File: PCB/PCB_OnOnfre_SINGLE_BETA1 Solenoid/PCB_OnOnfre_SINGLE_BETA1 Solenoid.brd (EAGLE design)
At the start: 44.1 x 43.8 mm, 32 parts, among them J1 9PIN 2.54MM, J3Y S8050, J7 8p, K1 G5Q-1-DC12, K2 G5Q-1-DC12, U2 esp12

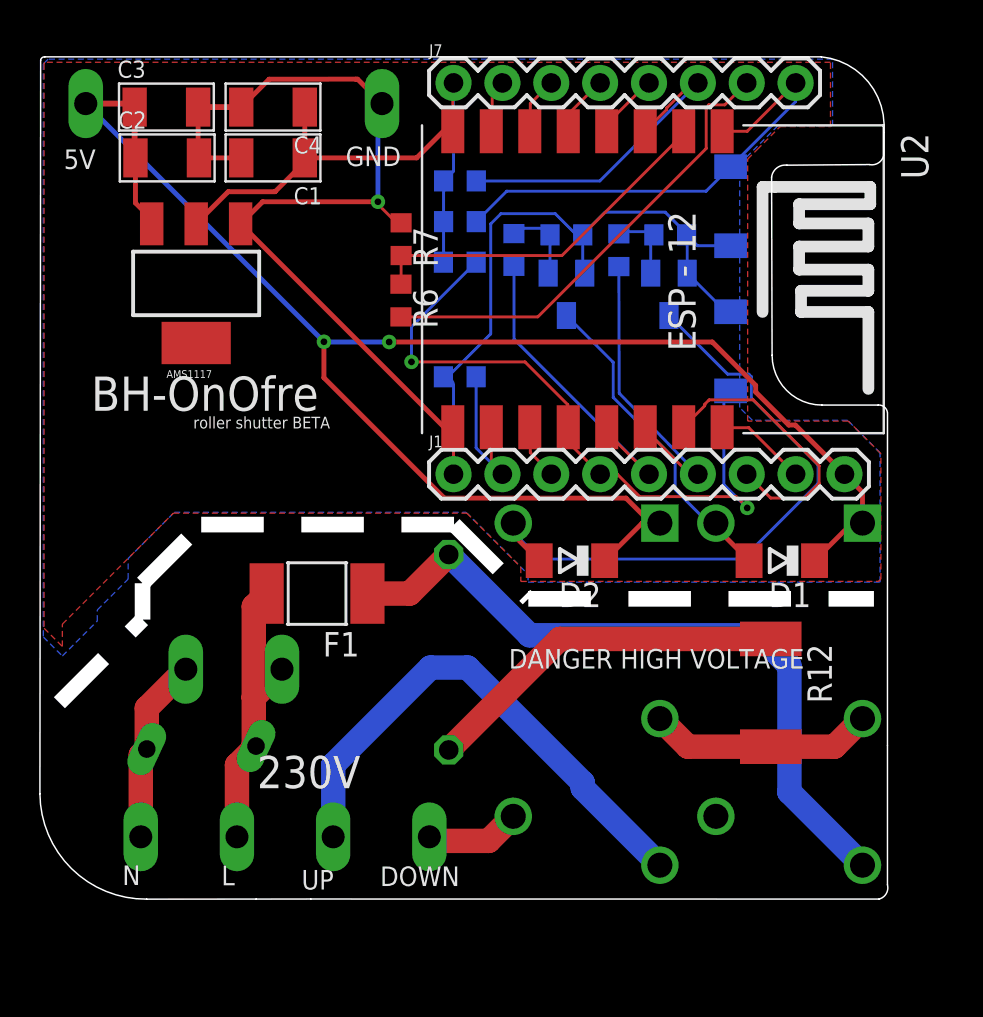
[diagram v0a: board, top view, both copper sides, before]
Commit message: bl
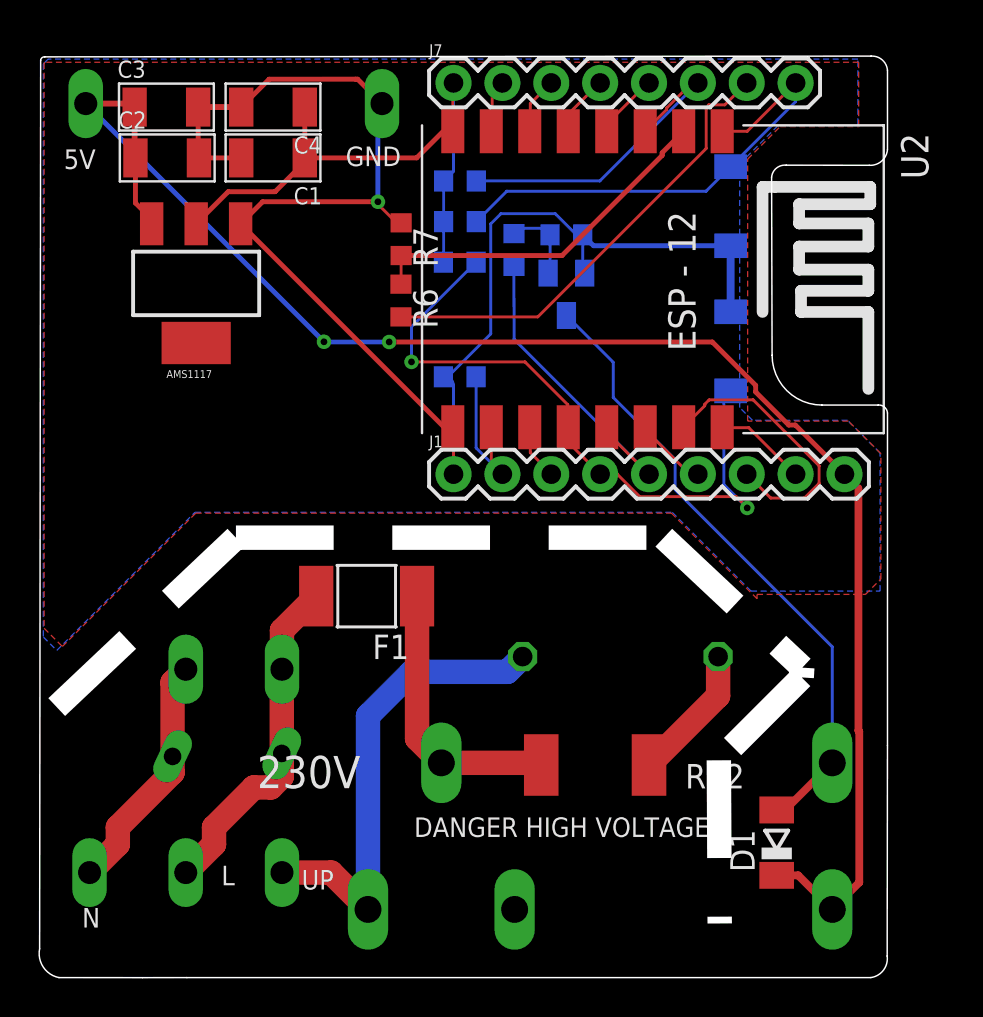
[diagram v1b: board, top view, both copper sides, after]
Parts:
- removed D2: 1N4148, diode:SOD80C
- removed JY3: S8050, semicon-smd-ipc:SOT23
- removed K1: G5Q-1-DC12, G5Q-1-DC12:RELAY_G5Q-1-DC12
- removed R1, R2: 10k, resistor:R0603
- removed X1: (no value), con-wago-500:W237-4
- added X2: (no value), con-wago-500:W237-103
- C1, C2: value 1NF -> 22uF
- C3, C4: value 1NF -> 100uF
- K2: value G5Q-1-DC12 -> E3206S; device G5Q-1-DC12:RELAY_G5Q-1-DC12 -> relay:E3206S
- moved D1 14.7 mm to (38.9, 5.48), turned to 90 degrees
- moved K2 12.2 mm to (38.7, 5.82), turned to 0 degrees
- moved R12 9.87 mm to (29.5, 9.52), turned to 180 degrees
- moved C6 8.92 mm to (30.8, 15.2), turned to 180 degrees
- moved F1 2.58 mm to (17.6, 18.3)
- moved R5 1.39 mm to (10.4, 10.0)
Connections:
- removed net LINE_DOWN_OUT: K2.4, X1.4
- removed net LINE_UP_OUT: K2.3, X1.3
- removed net N$13: JY3.1, R1.2, R2.2
- removed net N$3: K1.2, K2.2, R12.2
- removed net N$9: D2.A, JY3.3, K2.5
- new net LINE_OUT: C6.1, K2.S, X2.3
- net GND: no longer JY3.2, R2.1
- net GPIO05: no longer R1.1
- net LINE_IN_FUSED: now also K2.P, R12.2; no longer C6.1, K1.3
- net LINE_L: now also X2.2; no longer X1.2
- net N$1: now also K2.1; no longer K1.5
- net NEUTRAL_IN: now also X2.1; no longer X1.1
- net VCC: now also K2.2; no longer D2.C, K1.1, K2.1
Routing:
- net N$9: track 33.6 -> 0.00 mm
- net LINE_UP_OUT: track 27.2 -> 0.00 mm
- net LINE_OUT: track 0.00 -> 24.6 mm
- net LINE_IN_FUSED: track 37.1 -> 14.4 mm
- net N$1: track 16.9 -> 32.9 mm
- net GPIO05: track 16.3 -> 3.85 mm
- net N$5: track 19.1 -> 7.12 mm
- net N$3: track 11.7 -> 0.00 mm
- net VCC: track 89.7 -> 84.4 mm
- net LINE_DOWN_OUT: track 4.98 -> 0.00 mm
- net N$13: track 4.10 -> 0.00 mm
- net NEUTRAL_IN: track 9.68 -> 12.6 mm
- net GND: track 84.6 -> 81.8 mm
- net LINE_L: track 15.5 -> 17.7 mm
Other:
- board size 44.1 x 43.8 mm -> 44.1 x 47.9 mm
- board text removed: "BH-OnOfre"
- board text removed: "DOWN"
- board text removed: "roller shutter BETA"
